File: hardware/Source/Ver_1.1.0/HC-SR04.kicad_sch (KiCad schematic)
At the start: 0 parts

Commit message: update pcb v1.1.0
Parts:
- added C37: 10uF, automative_hexapod:Ceramic_Cap_0805, symbol automative_hexapod:Ceramic_Cap_0805_10uF_16V
- added C38: 100nF, automative_hexapod:Ceramic_Cap_0805, symbol automative_hexapod:Ceramic_Cap_0805_100nF_50V
- added J6: Connector, automative_hexapod:JST-XH-SMD-4-2.54mm, symbol automative_hexapod:JST-XH-SMD-4-2.54mm
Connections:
- new net +5V: C37.2, C38.2, J6.1 (Pin_1)
- new net GND: C37.1, C38.1, J6.4 (Pin_4)
- new net HCSR04_ECHO: J6.3 (Pin_3)
- new net HCSR04_TRIG: J6.2 (Pin_2)
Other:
- title: (none) -> HC-SR04

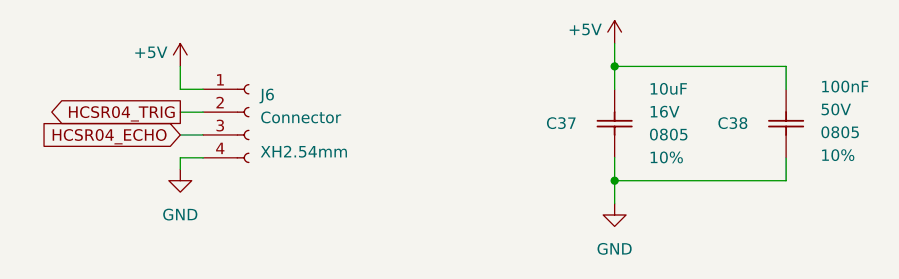
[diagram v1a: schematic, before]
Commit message: update pcb and schematic
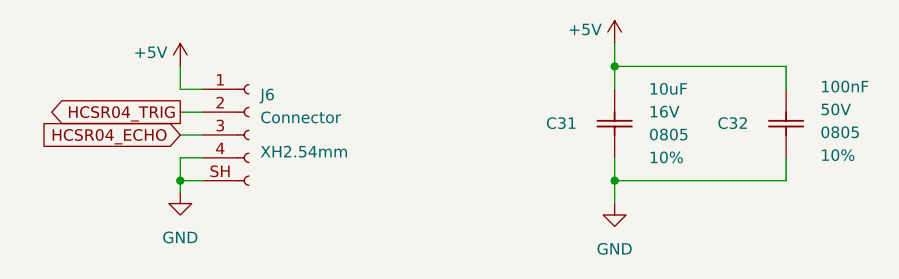
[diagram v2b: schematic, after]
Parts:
- renumbered C37 to C31, C38 to C32
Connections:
- net GND: now also J6.SH (Pin_3)
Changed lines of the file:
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@@
+	)
+	(junction
+		(at 128.27 86.36)
+		(diameter 0)
+		(color 0 0 0 0)
 	)
 	(junction
@@
 	(wire
 		(pts
+			(xy 128.27 86.36) (xy 130.81 86.36)
+		)
+		(stroke
+			(width 0)
+			(type default)
+		)
+	)
+	(wire
+		(pts
 			(xy 195.58 73.66) (xy 176.53 73.66)
 		)
@@
 	(wire
 		(pts
-			(xy 128.27 83.82) (xy 128.27 85.09)
+			(xy 128.27 83.82) (xy 128.27 86.36)
 		)
 		(stroke
@@
 		(pts
 			(xy 128.27 81.28) (xy 130.81 81.28)
+		)
+		(stroke
+			(width 0)
+			(type default)
+		)
+	)
+	(wire
+		(pts
+			(xy 128.27 86.36) (xy 128.27 87.63)
 		)
 		(stroke
@@
 		(on_board yes)
 		(dnp no)
-		(property "Reference" "C38"
+		(property "Reference" "C32"
 			(at 187.96 80.01 90)
 			(effects
@@
 			(project "Automative_Hexapod"
 				(path "/c07b6013-2147-4cef-a16e-342deb9ccbf5/716aec1c-0009-4d7b-ab53-21c905b5927d"
-					(reference "C38")
+					(reference "C32")
 					(unit 1)
 				)
@@
 	(symbol
 		(lib_id "power:GND")
-		(at 128.27 85.09 0)
+		(at 128.27 87.63 0)
 		(unit 1)
 		(exclude_from_sim no)
@@
 		(dnp no)
 		(fields_autoplaced yes)
-		(property "Reference" "#PWR094"
-			(at 128.27 91.44 0)
+		(property "Reference" "#PWR093"
+			(at 128.27 93.98 0)
 			(effects
 				(font
@@
 		)
 		(property "Value" "GND"
-			(at 128.27 90.17 0)
+			(at 128.27 92.71 0)
 			(effects
 				(font
@@
 		)
 		(property "Footprint" ""
-			(at 128.27 85.09 0)
+			(at 128.27 87.63 0)
 			(effects
 				(font
@@
 		)
 		(property "Datasheet" ""
-			(at 128.27 85.09 0)
+			(at 128.27 87.63 0)
 			(effects
 				(font
@@
 		)
 		(property "Description" "Power symbol creates a global label with name \"GND\" , ground"
-			(at 128.27 85.09 0)
+			(at 128.27 87.63 0)
 			(effects
 				(font
@@
 			(project "Automative_Hexapod"
 				(path "/c07b6013-2147-4cef-a16e-342deb9ccbf5/716aec1c-0009-4d7b-ab53-21c905b5927d"
-					(reference "#PWR094")
+					(reference "#PWR093")
 					(unit 1)
 				)
@@
 		(pin "3"
 		)
+		(pin "SH"
+		)
 		(instances
 			(project ""
@@
 		(dnp no)
 		(fields_autoplaced yes)
-		(property "Reference" "#PWR096"
+		(property "Reference" "#PWR095"
 			(at 176.53 95.25 0)
 			(effects
@@
 			(project "Automative_Hexapod"
 				(path "/c07b6013-2147-4cef-a16e-342deb9ccbf5/716aec1c-0009-4d7b-ab53-21c905b5927d"
-					(reference "#PWR096")
+					(reference "#PWR095")
 					(unit 1)
 				)
@@
 		(on_board yes)
 		(dnp no)
-		(property "Reference" "#PWR095"
+		(property "Reference" "#PWR094"
 			(at 176.53 74.93 0)
 			(effects
@@
 			(project "Automative_Hexapod"
 				(path "/c07b6013-2147-4cef-a16e-342deb9ccbf5/716aec1c-0009-4d7b-ab53-21c905b5927d"
-					(reference "#PWR095")
+					(reference "#PWR094")
 					(unit 1)
 				)
@@
 		(on_board yes)
 		(dnp no)
-		(property "Reference" "C37"
+		(property "Reference" "C31"
 			(at 168.91 80.01 90)
 			(effects
@@
 			(project "Automative_Hexapod"
 				(path "/c07b6013-2147-4cef-a16e-342deb9ccbf5/716aec1c-0009-4d7b-ab53-21c905b5927d"
-					(reference "C37")
+					(reference "C31")
 					(unit 1)
 				)
@@
 		(on_board yes)
 		(dnp no)
-		(property "Reference" "#PWR093"
+		(property "Reference" "#PWR092"
 			(at 128.27 77.47 0)
 			(effects
@@
 			(project "Automative_Hexapod"
 				(path "/c07b6013-2147-4cef-a16e-342deb9ccbf5/716aec1c-0009-4d7b-ab53-21c905b5927d"
-					(reference "#PWR093")
+					(reference "#PWR092")
 					(unit 1)
 				)
